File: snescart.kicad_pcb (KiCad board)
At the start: 2 copper layers, 101.6 x 37.3 mm, 7 parts, among them P1 CASSETTE, U1 27C080

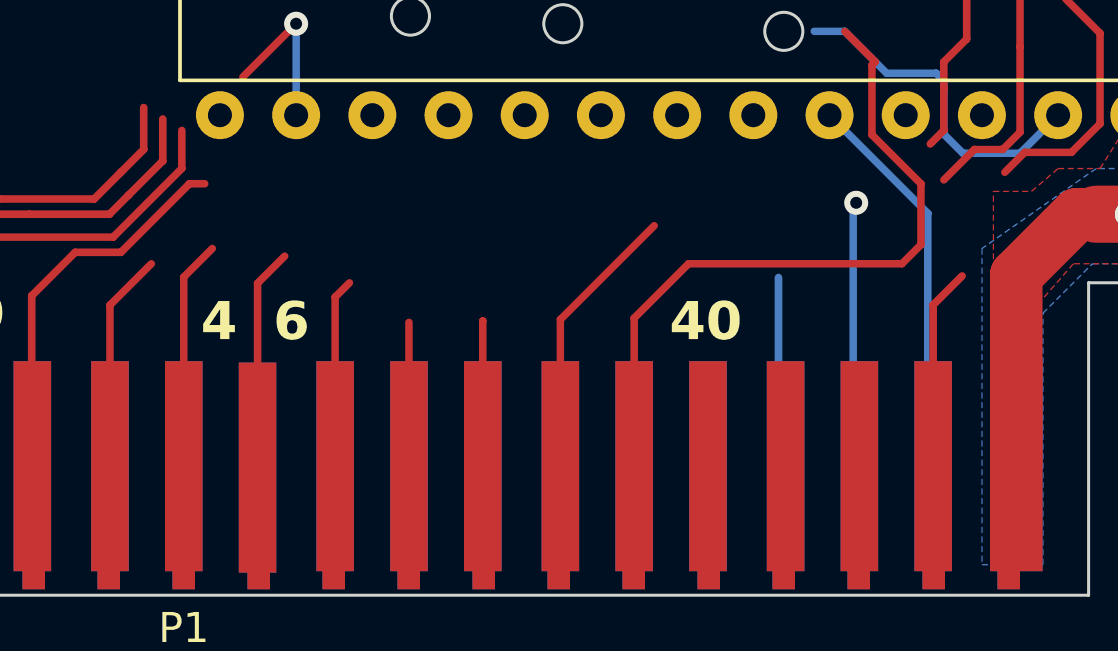
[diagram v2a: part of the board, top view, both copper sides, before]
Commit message: Update snescart.kicad_pcb
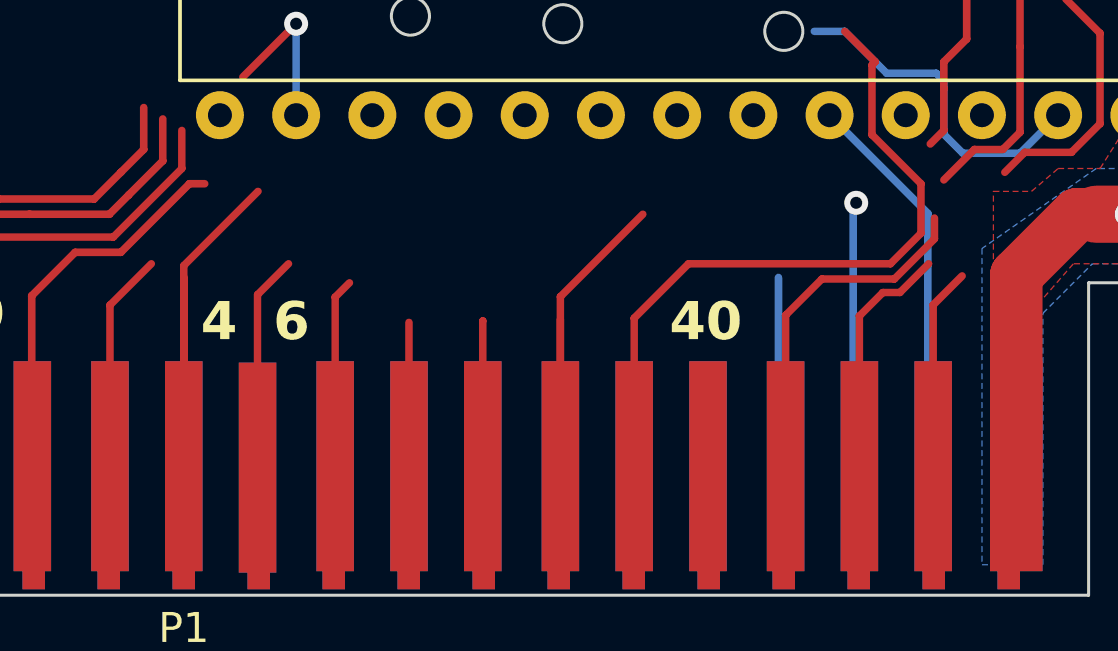
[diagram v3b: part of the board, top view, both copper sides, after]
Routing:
- net Net-(P1-A14): track 6.55 -> 18.3 mm
- net unconnected-(P1-A22-Pad47): track 7.65 -> 16.5 mm
- net Net-(P1-A13): track 21.8 -> 29.9 mm
- net Net-(P1-A17): track 9.31 -> 14.4 mm
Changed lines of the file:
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@@
   (segment (start 171.323 128.524) (end 171.323 127.762) (width 0.25) (layer "F.Cu") (net 36))
   (segment (start 172.72 134.427991) (end 172.146991 135.001) (width 0.25) (layer "F.Cu") (net 36))
+  (segment (start 167.365 145.559) (end 167.365 140.552) (width 0.25) (layer "F.Cu") (net 36))
+  (segment (start 168.148 139.769) (end 168.716792 139.769) (width 0.25) (layer "F.Cu") (net 36))
+  (segment (start 168.716792 139.769) (end 169.673396 138.812396) (width 0.25) (layer "F.Cu") (net 36))
   (segment (start 172.72 129.921) (end 171.958 129.159) (width 0.25) (layer "F.Cu") (net 36))
+  (segment (start 167.365 140.552) (end 168.148 139.769) (width 0.25) (layer "F.Cu") (net 36))
   (segment (start 173.99 133.858) (end 172.72 135.128) (width 0.25) (layer "B.Cu") (net 36))
   (segment (start 168.275 132.461) (end 166.878 131.064) (width 0.25) (layer "B.Cu") (net 36))
@@
   (segment (start 170.18 134.493) (end 170.18 132.715) (width 0.25) (layer "B.Cu") (net 36))
   (segment (start 170.18 132.969) (end 170.18 132.08) (width 0.254) (layer "F.Cu") (net 37))
+  (segment (start 164.905 145.559) (end 164.905 140.53) (width 0.25) (layer "F.Cu") (net 37))
   (segment (start 170.942 131.318) (end 170.942 129.667) (width 0.254) (layer "F.Cu") (net 37))
   (segment (start 170.18 134.366) (end 170.18 132.969) (width 0.254) (layer "F.Cu") (net 37))
+  (segment (start 166.116 139.319) (end 168.530396 139.319) (width 0.25) (layer "F.Cu") (net 37))
   (segment (start 169.728 134.818) (end 170.18 134.366) (width 0.254) (layer "F.Cu") (net 37))
+  (segment (start 169.868 137.981396) (end 169.868 137.287) (width 0.25) (layer "F.Cu") (net 37))
   (segment (start 170.18 132.08) (end 170.942 131.318) (width 0.254) (layer "F.Cu") (net 37))
   (segment (start 170.942 129.667) (end 170.307 129.032) (width 0.254) (layer "F.Cu") (net 37))
-  (segment (start 161.671 138.811) (end 168.783 138.811) (width 0.25) (layer "F.Cu") (net 39))
+  (segment (start 168.530396 139.319) (end 169.868 137.981396) (width 0.25) (layer "F.Cu") (net 37))
+  (segment (start 164.905 140.53) (end 166.116 139.319) (width 0.25) (layer "F.Cu") (net 37))
+  (segment (start 169.418 137.795) (end 169.418 136.144) (width 0.25) (layer "F.Cu") (net 39))
   (segment (start 167.785 132.189) (end 167.894 132.08) (width 0.25) (layer "F.Cu") (net 39))
   (segment (start 167.785 134.511) (end 167.785 132.189) (width 0.25) (layer "F.Cu") (net 39))
-  (segment (start 168.783 138.811) (end 169.418 138.176) (width 0.25) (layer "F.Cu") (net 39))
-  (segment (start 169.418 138.176) (end 169.418 136.144) (width 0.25) (layer "F.Cu") (net 39))
   (segment (start 159.858 140.624) (end 161.671 138.811) (width 0.25) (layer "F.Cu") (net 39))
   (segment (start 159.858 145.559) (end 159.858 140.624) (width 0.25) (layer "F.Cu") (net 39))
   (segment (start 167.894 132.08) (end 166.878 131.064) (width 0.25) (layer "F.Cu") (net 39))
+  (segment (start 161.671 138.811) (end 168.402 138.811) (width 0.25) (layer "F.Cu") (net 39))
+  (segment (start 168.402 138.811) (end 169.418 137.795) (width 0.25) (layer "F.Cu") (net 39))
   (segment (start 169.418 136.144) (end 167.785 134.511) (width 0.25) (layer "F.Cu") (net 39))
+  (segment (start 157.398 145.559) (end 157.398 139.909) (width 0.25) (layer "F.Cu") (net 40))
   (segment (start 157.398 145.559) (end 157.398 140.671) (width 0.25) (layer "F.Cu") (net 40))
-  (segment (start 157.398 140.671) (end 160.528 137.541) (width 0.25) (layer "F.Cu") (net 40))
+  (segment (start 157.398 139.909) (end 160.147 137.16) (width 0.25) (layer "F.Cu") (net 40))
   (segment (start 154.811 140.718) (end 154.813 140.716) (width 0.25) (layer "F.Cu") (net 41))
   (segment (start 154.811 145.559) (end 154.811 140.718) (width 0.25) (layer "F.Cu") (net 41))
@@
   (segment (start 149.891 145.559) (end 149.891 139.923) (width 0.25) (layer "F.Cu") (net 52))
   (segment (start 149.891 139.923) (end 150.368 139.446) (width 0.25) (layer "F.Cu") (net 52))
-  (segment (start 147.304 145.607) (end 147.304 139.462) (width 0.25) (layer "F.Cu") (net 53))
-  (segment (start 147.304 139.462) (end 148.209 138.557) (width 0.25) (layer "F.Cu") (net 53))
-  (segment (start 144.844 139.255) (end 145.796 138.303) (width 0.25) (layer "F.Cu") (net 54))
+  (segment (start 147.304 139.843) (end 148.336 138.811) (width 0.25) (layer "F.Cu") (net 53))
+  (segment (start 147.304 145.607) (end 147.304 139.843) (width 0.25) (layer "F.Cu") (net 53))
+  (segment (start 144.844 145.559) (end 144.844 138.874) (width 0.25) (layer "F.Cu") (net 54))
+  (segment (start 144.844 138.874) (end 147.32 136.398) (width 0.25) (layer "F.Cu") (net 54))
   (segment (start 144.844 145.559) (end 144.844 139.255) (width 0.25) (layer "F.Cu") (net 54))
   (segment (start 142.384 140.191) (end 143.764 138.811) (width 0.25) (layer "F.Cu") (net 55))
